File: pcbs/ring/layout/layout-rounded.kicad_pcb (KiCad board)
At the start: 2 copper layers, 57 x 6.2 mm, 65 parts, among them J1 ?, Q1 CSD13380F3T, Q2 CSD13380F3T, U1 BQ27427YZFR, U2 BQ29700, U3 nRF52833-QDAA, U4 MAX30102EFD+T, U5 LSM6DSOX, U6 TMP117AIDRVR, U7 TPS7A2018PDQN, Y1 32MHz, Y2 32.768kHz

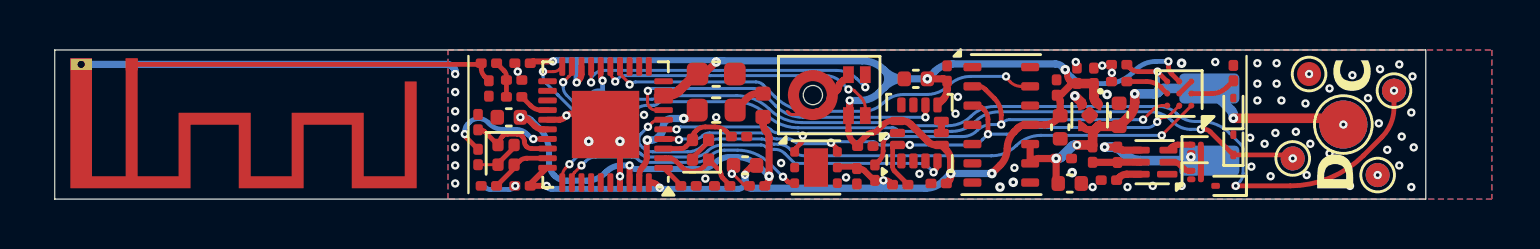
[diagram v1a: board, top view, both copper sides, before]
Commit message: cleanup
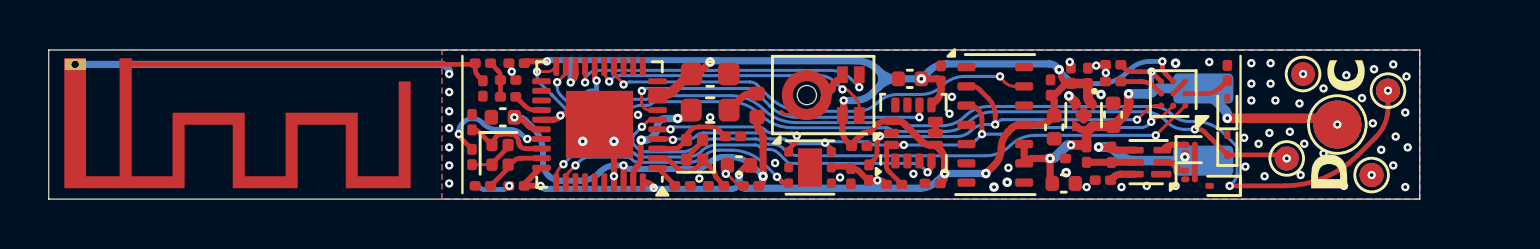
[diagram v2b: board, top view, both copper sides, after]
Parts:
- moved BT1 0.25 mm to (166.0, 83.1)
- moved C1 0.25 mm to (162.3, 80.6)
- moved C10 0.25 mm to (145.8, 85.7)
- moved C11 0.25 mm to (146.4, 83.6)
- moved C12 0.25 mm to (144.3, 85.7)
- moved C13 0.25 mm to (135.6, 84.5)
- moved C14 0.25 mm to (136.9, 82.8)
- moved C15 0.25 mm to (147.2, 85.7)
- moved C16 0.25 mm to (137.1, 81.2)
- moved C17 0.25 mm to (136.1, 81.6)
- moved C18 0.25 mm to (160.2, 85.5)
- moved C19 0.25 mm to (160.0, 84.5)
- moved C2 0.25 mm to (162.3, 81.3)
- moved C20 0.25 mm to (159.8, 83.2)
- moved C21 0.25 mm to (159.7, 81.6)
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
